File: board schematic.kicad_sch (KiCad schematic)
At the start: 26 parts, among them SW1 E-Stop Button, U1 ESP32-S3-WROOM-1-N16R8

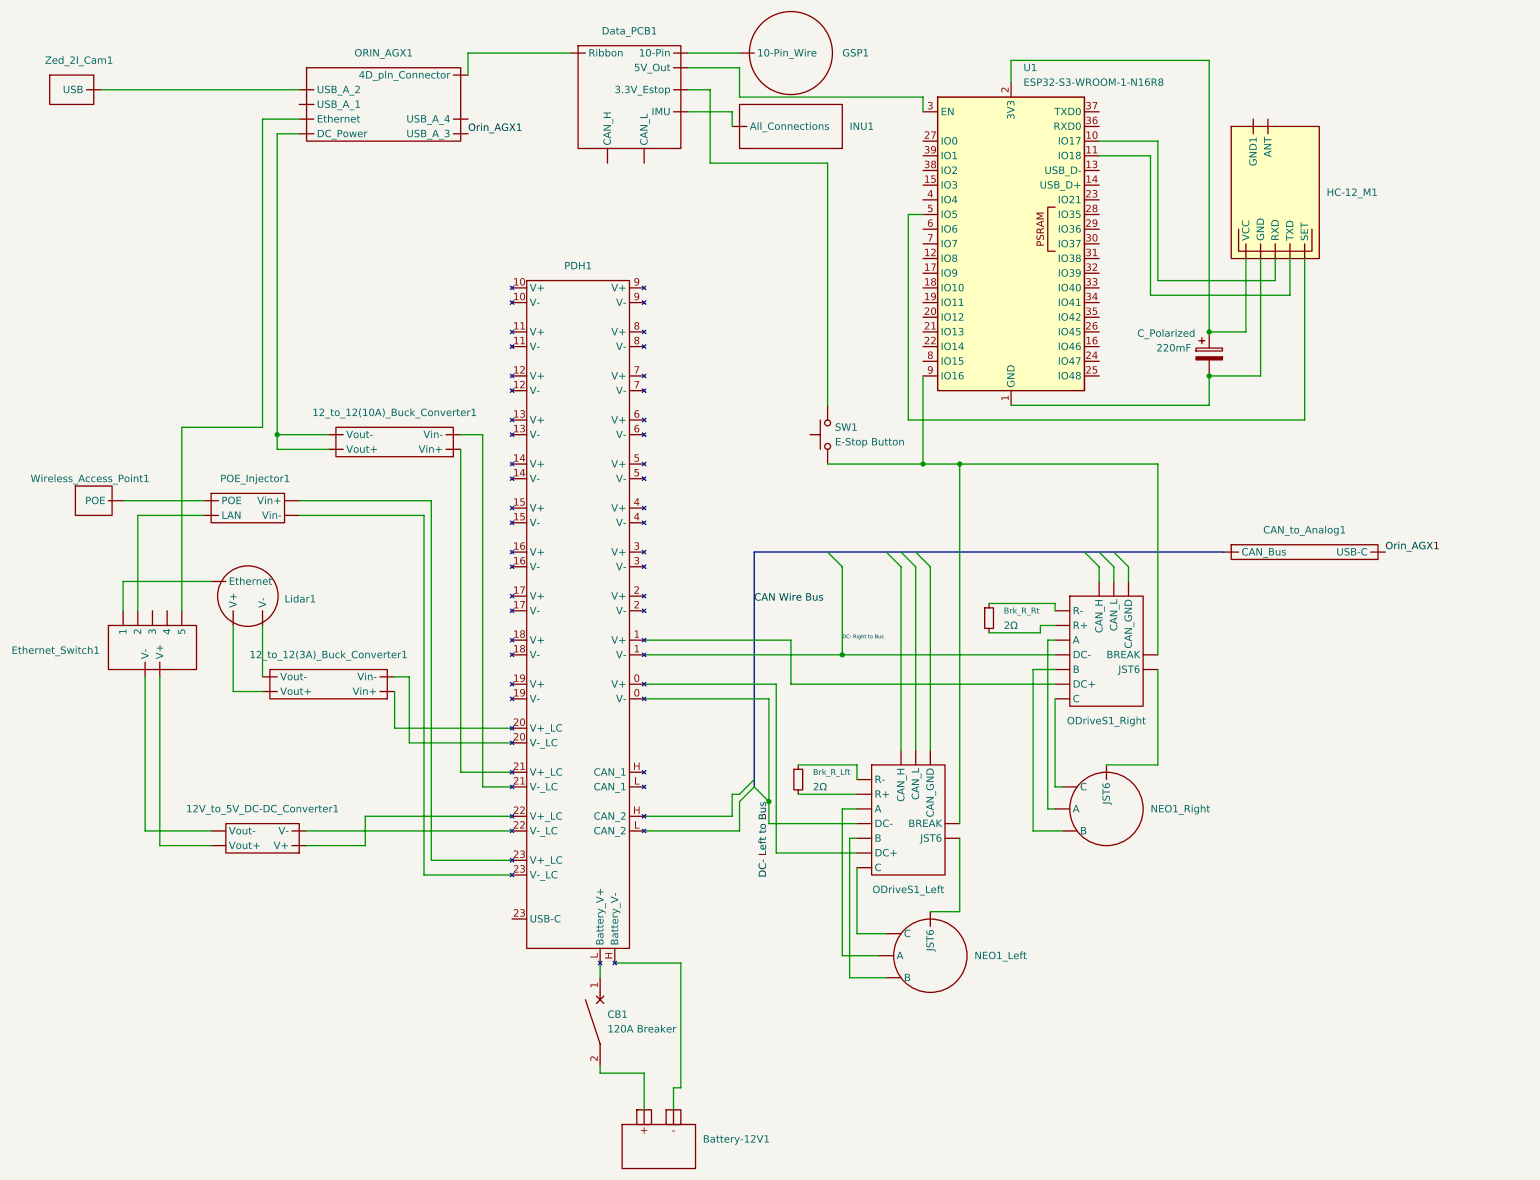
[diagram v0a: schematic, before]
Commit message: Schematic 1 Updated
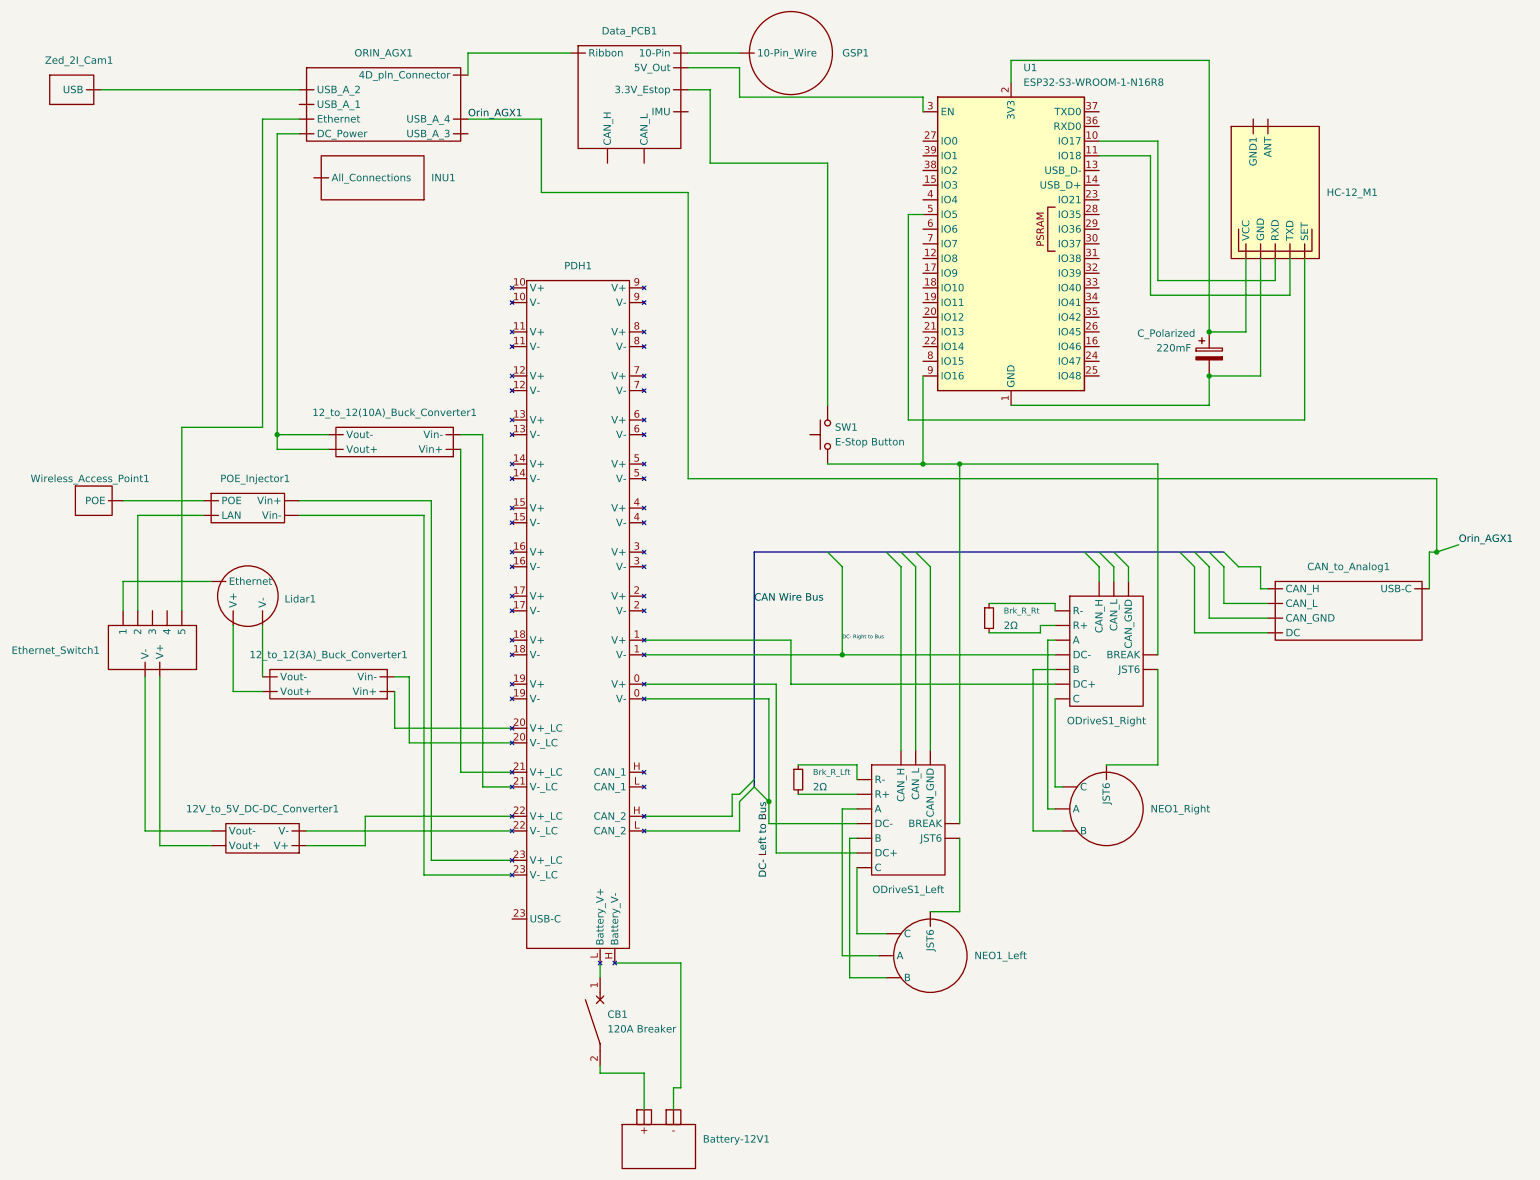
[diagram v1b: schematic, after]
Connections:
- net at POE_Injector1. (Vin-): now also Ethernet_Switch1. (5); no longer PDH1.23 (USB-C)
- net at PDH1.23 (USB-C): no longer POE_Injector1. (Vin-)
- net at Ethernet_Switch1. (5): now also ORIN_AGX1. (USB_A_3); no longer POE_Injector1. (Vin-)
- net at 12_to_12(3A)_Buck_Converter1. (Vout-): now also Lidar1. (V-); no longer PDH1.20 (V-_LC)
- net at 12_to_12(10A)_Buck_Converter1. (Vout-): now also ORIN_AGX1. (USB_A_3); no longer PDH1.21 (V-_LC)
- net at 12V_to_5V_DC-DC_Converter1. (Vout-): now also Ethernet_Switch1. (5); no longer PDH1.22 (V-_LC)
- net at PDH1.H (CAN_2): now also Battery-12V1.
- net at Battery-12V1.: now also CB1.2; no longer PDH1.H (CAN_2)
- net at PDH1.L (CAN_2): now also CB1.1
- net at INU1. (All_Connections): no longer Data_PCB1. (IMU)
- net at Data_PCB1. (IMU): now also ORIN_AGX1. (USB_A_3)
- new net: PDH1.23 (USB-C), POE_Injector1. (Vin-) (x2)
- new net: ODriveS1_Left. (JST6), PDH1.0 (V-)
- new net: ODriveS1_Right. (JST6), PDH1.1 (V-)
- new net: 12_to_12(3A)_Buck_Converter1. (Vout-), PDH1.20 (V-_LC)
- new net: 12_to_12(10A)_Buck_Converter1. (Vout-), PDH1.21 (V-_LC)
- new net: 12V_to_5V_DC-DC_Converter1. (Vout-), PDH1.22 (V-_LC)
- new net: NEO1_Right. (JST6), ODriveS1_Right. (JST6) (x3)
- new net: 12V_to_5V_DC-DC_Converter1. (Vout-), Ethernet_Switch1. (5)
- new net: Ethernet_Switch1. (5), Lidar1. (V-)
- new net: NEO1_Left. (JST6), ODriveS1_Left. (JST6) (x3)
- new net: 12_to_12(3A)_Buck_Converter1. (Vout-), Lidar1. (V-)
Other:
- moved on the sheet: INU1
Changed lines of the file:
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@@
 	)
 	(junction
+		(at 273.05 105.41)
+		(diameter 0)
+		(color 0 0 0 0)
+	)
+	(junction
 		(at 170.18 123.19)
 		(diameter 0)
@@
 	)
 	(bus_entry
+		(at 231.14 105.41)
+		(size 2.54 2.54)
+		(stroke
+			(width 0)
+			(type default)
+		)
+	)
+	(bus_entry
+		(at 228.6 105.41)
+		(size 2.54 2.54)
+		(stroke
+			(width 0)
+			(type default)
+		)
+	)
+	(bus_entry
+		(at 236.22 105.41)
+		(size 2.54 2.54)
+		(stroke
+			(width 0)
+			(type default)
+		)
+	)
+	(bus_entry
 		(at 152.4 147.32)
 		(size 2.54 -2.54)
@@
 	)
 	(bus_entry
+		(at 233.68 105.41)
+		(size 2.54 2.54)
+		(stroke
+			(width 0)
+			(type default)
+		)
+	)
+	(bus_entry
 		(at 180.34 105.41)
 		(size 2.54 2.54)
@@
 	(wire
 		(pts
+			(xy 242.57 107.95) (xy 238.76 107.95)
+		)
+		(stroke
+			(width 0)
+			(type default)
+		)
+	)
+	(wire
+		(pts
 			(xy 95.25 138.43) (xy 95.25 127)
 		)
@@
 	(wire
 		(pts
+			(xy 236.22 114.3) (xy 236.22 107.95)
+		)
+		(stroke
+			(width 0)
+			(type default)
+		)
+	)
+	(wire
+		(pts
 			(xy 250.19 82.55) (xy 250.19 54.61)
 		)
@@
 	(wire
 		(pts
+			(xy 243.84 114.3) (xy 236.22 114.3)
+		)
+		(stroke
+			(width 0)
+			(type default)
+		)
+	)
+	(wire
+		(pts
 			(xy 142.24 176.53) (xy 142.24 198.12)
 		)
@@
 	(wire
 		(pts
+			(xy 233.68 116.84) (xy 243.84 116.84)
+		)
+		(stroke
+			(width 0)
+			(type default)
+		)
+	)
+	(wire
+		(pts
 			(xy 113.03 158.75) (xy 99.06 158.75)
 		)
@@
 	(wire
 		(pts
+			(xy 273.05 105.41) (xy 273.05 92.71)
+		)
+		(stroke
+			(width 0)
+			(type default)
+		)
+	)
+	(wire
+		(pts
 			(xy 207.01 115.57) (xy 207.01 114.3)
 		)
@@
 	(wire
 		(pts
+			(xy 242.57 111.76) (xy 243.84 111.76)
+		)
+		(stroke
+			(width 0)
+			(type default)
+		)
+	)
+	(wire
+		(pts
 			(xy 72.39 33.02) (xy 76.2 33.02)
 		)
@@
 	(wire
 		(pts
+			(xy 233.68 107.95) (xy 233.68 116.84)
+		)
+		(stroke
+			(width 0)
+			(type default)
+		)
+	)
+	(wire
+		(pts
+			(xy 271.78 111.76) (xy 271.78 105.41)
+		)
+		(stroke
+			(width 0)
+			(type default)
+		)
+	)
+	(wire
+		(pts
 			(xy 135.89 120.65) (xy 161.29 120.65)
 		)
@@
 	(wire
 		(pts
+			(xy 118.11 30.48) (xy 105.41 30.48)
+		)
+		(stroke
+			(width 0)
+			(type default)
+		)
+	)
+	(wire
+		(pts
 			(xy 147.32 38.1) (xy 147.32 25.4)
 		)
@@
 	(wire
 		(pts
-			(xy 151.13 29.21) (xy 151.13 31.75)
+			(xy 140.97 198.12) (xy 140.97 201.93)
 		)
 		(stroke
@@
 	(wire
 		(pts
-			(xy 140.97 198.12) (xy 140.97 201.93)
+			(xy 81.28 87.63) (xy 72.39 87.63)
 		)
 		(stroke
@@
 	(wire
 		(pts
-			(xy 81.28 87.63) (xy 72.39 87.63)
+			(xy 172.72 149.86) (xy 170.18 149.86)
 		)
 		(stroke
@@
 	(wire
 		(pts
-			(xy 172.72 149.86) (xy 170.18 149.86)
+			(xy 247.65 54.61) (xy 247.65 60.96)
 		)
 		(stroke
@@
 	(wire
 		(pts
-			(xy 247.65 54.61) (xy 247.65 60.96)
+			(xy 271.78 105.41) (xy 273.05 105.41)
 		)
 		(stroke
@@
 	(wire
 		(pts
+			(xy 273.05 92.71) (xy 143.51 92.71)
+		)
+		(stroke
+			(width 0)
+			(type default)
+		)
+	)
+	(wire
+		(pts
 			(xy 158.75 128.27) (xy 158.75 157.48)
 		)
@@
 	(wire
 		(pts
+			(xy 118.11 43.18) (xy 118.11 30.48)
+		)
+		(stroke
+			(width 0)
+			(type default)
+		)
+	)
+	(wire
+		(pts
 			(xy 97.79 99.06) (xy 97.79 161.29)
 		)
@@
 	(wire
 		(pts
+			(xy 143.51 43.18) (xy 118.11 43.18)
+		)
+		(stroke
+			(width 0)
+			(type default)
+		)
+	)
+	(wire
+		(pts
 			(xy 167.64 80.01) (xy 167.64 38.1)
 		)
@@
 	(wire
 		(pts
+			(xy 231.14 119.38) (xy 231.14 107.95)
+		)
+		(stroke
+			(width 0)
+			(type default)
+		)
+	)
+	(wire
+		(pts
 			(xy 64.77 129.54) (xy 69.85 129.54)
 		)
@@
 		)
 	)
+	(wire
+		(pts
+			(xy 243.84 119.38) (xy 231.14 119.38)
+		)
+		(stroke
+			(width 0)
+			(type default)
+		)
+	)
 	(bus
 		(pts
@@
 	(wire
 		(pts
+			(xy 143.51 92.71) (xy 143.51 43.18)
+		)
+		(stroke
+			(width 0)
+			(type default)
+		)
+	)
+	(wire
+		(pts
 			(xy 245.11 58.42) (xy 245.11 54.61)
 		)
@@
 	(wire
 		(pts
+			(xy 276.86 104.14) (xy 273.05 105.41)
+		)
+		(stroke
+			(width 0)
+			(type default)
+		)
+	)
+	(wire
+		(pts
 			(xy 69.85 118.11) (xy 69.85 127)
 		)
@@
 	(wire
 		(pts
-			(xy 143.51 29.21) (xy 151.13 29.21)
+			(xy 81.28 85.09) (xy 72.39 85.09)
 		)
 		(stroke
@@
 	(wire
 		(pts
-			(xy 81.28 85.09) (xy 72.39 85.09)
+			(xy 233.68 80.01) (xy 233.68 74.93)
 		)
 		(stroke
@@
 	(wire
 		(pts
-			(xy 233.68 80.01) (xy 233.68 74.93)
+			(xy 224.79 58.42) (xy 245.11 58.42)
 		)
 		(stroke
@@
 	(wire
 		(pts
-			(xy 224.79 58.42) (xy 245.11 58.42)
+			(xy 242.57 111.76) (xy 242.57 107.95)
 		)
 		(stroke
@@
 	)
 	(label "Orin_AGX1"
-		(at 264.16 105.41 0)
+		(at 276.86 104.14 0)
 		(effects
 			(font
@@
 	)
 	(label "Orin_AGX1"
-		(at 105.41 33.02 0)
+		(at 105.41 30.48 0)
 		(effects
 			(font
@@
 	(symbol
 		(lib_id "IGVC-components:INU1")
-		(at 161.29 36.83 0)
+		(at 88.9 45.72 0)
 		(unit 1)
 		(body_style 1)
@@
 		(fields_autoplaced yes)
 		(property "Reference" "INU1"
-			(at 171.45 31.7499 0)
+			(at 99.06 40.6399 0)
 			(show_name no)
 			(do_not_autoplace no)
@@
 		)
 		(property "Value" ""
-			(at 161.29 36.83 0)
+			(at 88.9 45.72 0)
 			(show_name no)
 			(do_not_autoplace no)
@@
 		)
 		(property "Footprint" ""
-			(at 161.29 36.83 0)
+			(at 88.9 45.72 0)
 			(hide yes)
 			(show_name no)
@@
 		)
 		(property "Datasheet" ""
-			(at 161.29 36.83 0)
+			(at 88.9 45.72 0)
 			(hide yes)
 			(show_name no)
@@
 		)
 		(property "Description" ""
-			(at 161.29 36.83 0)
+			(at 88.9 45.72 0)
 			(hide yes)
 			(show_name no)
@@
 	(symbol
 		(lib_id "IGVC-components:CAN_to_Analog")
-		(at 250.19 109.22 0)
+		(at 257.81 115.57 0)
 		(unit 1)
 		(body_style 1)
@@
 		(fields_autoplaced yes)
 		(property "Reference" "CAN_to_Analog1"
-			(at 250.19 101.6 0)
+			(at 257.81 107.95 0)
 			(show_name no)
 			(do_not_autoplace no)
@@
 		)
 		(property "Value" ""
-			(at 250.19 109.22 0)
+			(at 257.81 115.57 0)
 			(show_name no)
 			(do_not_autoplace no)
@@
 		)
 		(property "Footprint" ""
-			(at 250.19 109.22 0)
+			(at 257.81 115.57 0)
 			(hide yes)
 			(show_name no)
@@
 		)
 		(property "Datasheet" ""
-			(at 250.19 109.22 0)
+			(at 257.81 115.57 0)
 			(hide yes)
 			(show_name no)
@@
 		)
 		(property "Description" ""
-			(at 250.19 109.22 0)
+			(at 257.81 115.57 0)
 			(hide yes)
 			(show_name no)
@@
 		)
 		(pin ""
+		)
+		(pin ""
+		)
+		(pin ""
+		)
+		(pin ""
